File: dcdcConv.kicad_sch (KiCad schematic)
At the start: 72 parts, among them J17 PWRSWITCH, J18 Conn_01x02, J19 EN, J20 Conn_01x03, J21 PGOOD, J22 Conn_01x03, U10 TLV62130, U7 TLV62130, U8 TLV62130, U9 MAX42402AFLB+

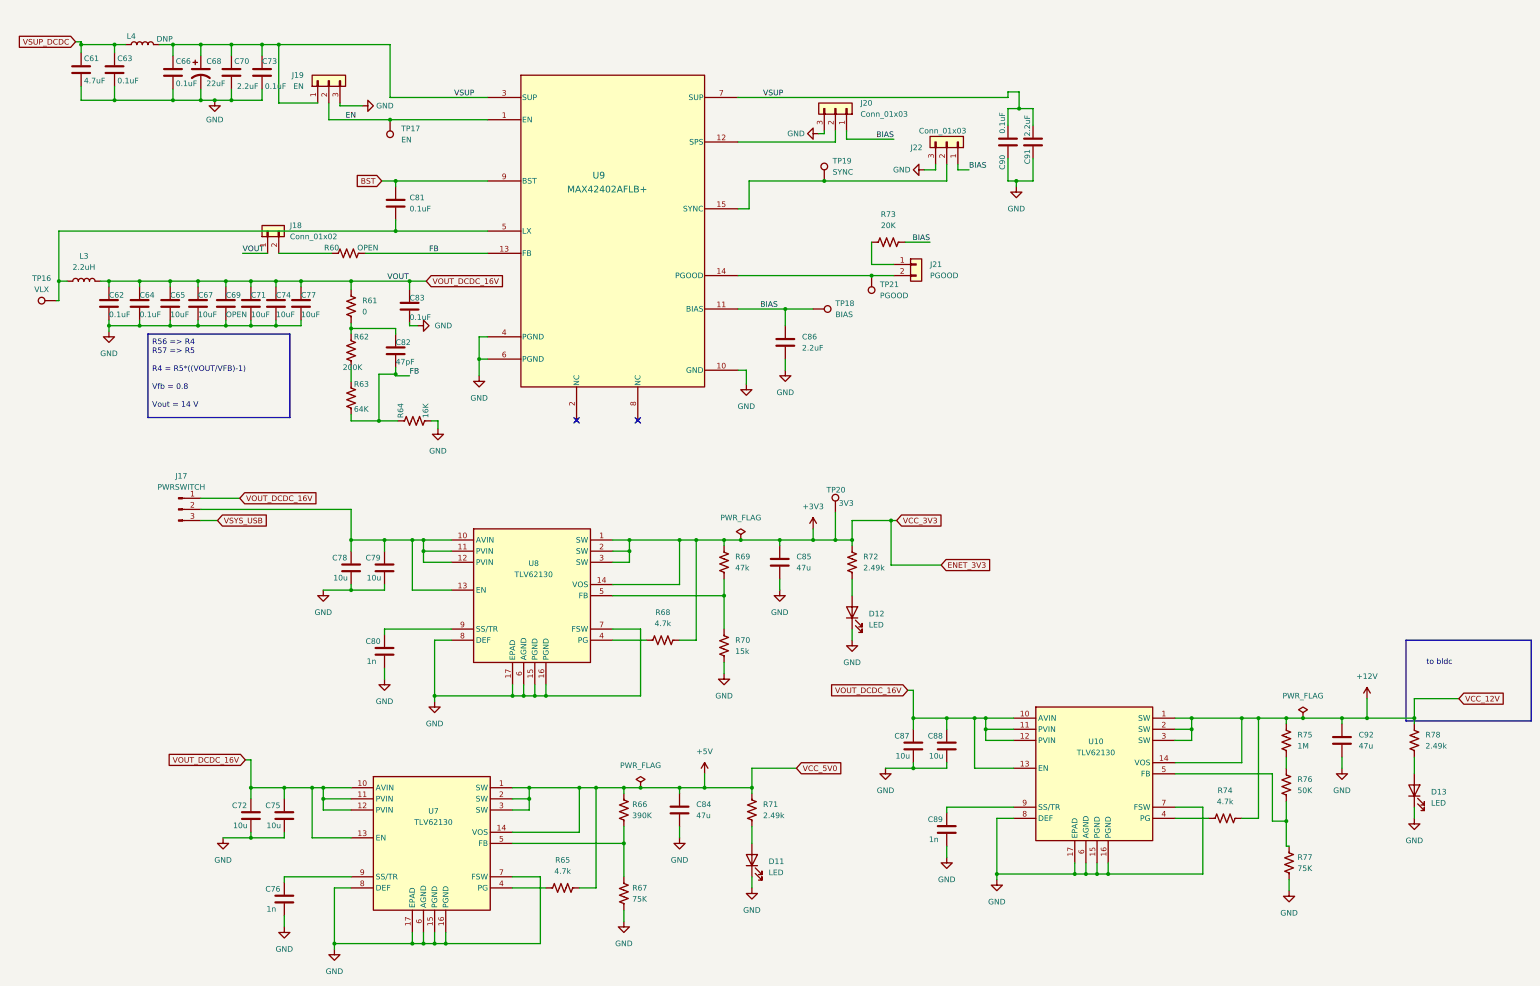
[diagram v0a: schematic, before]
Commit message: dad
da
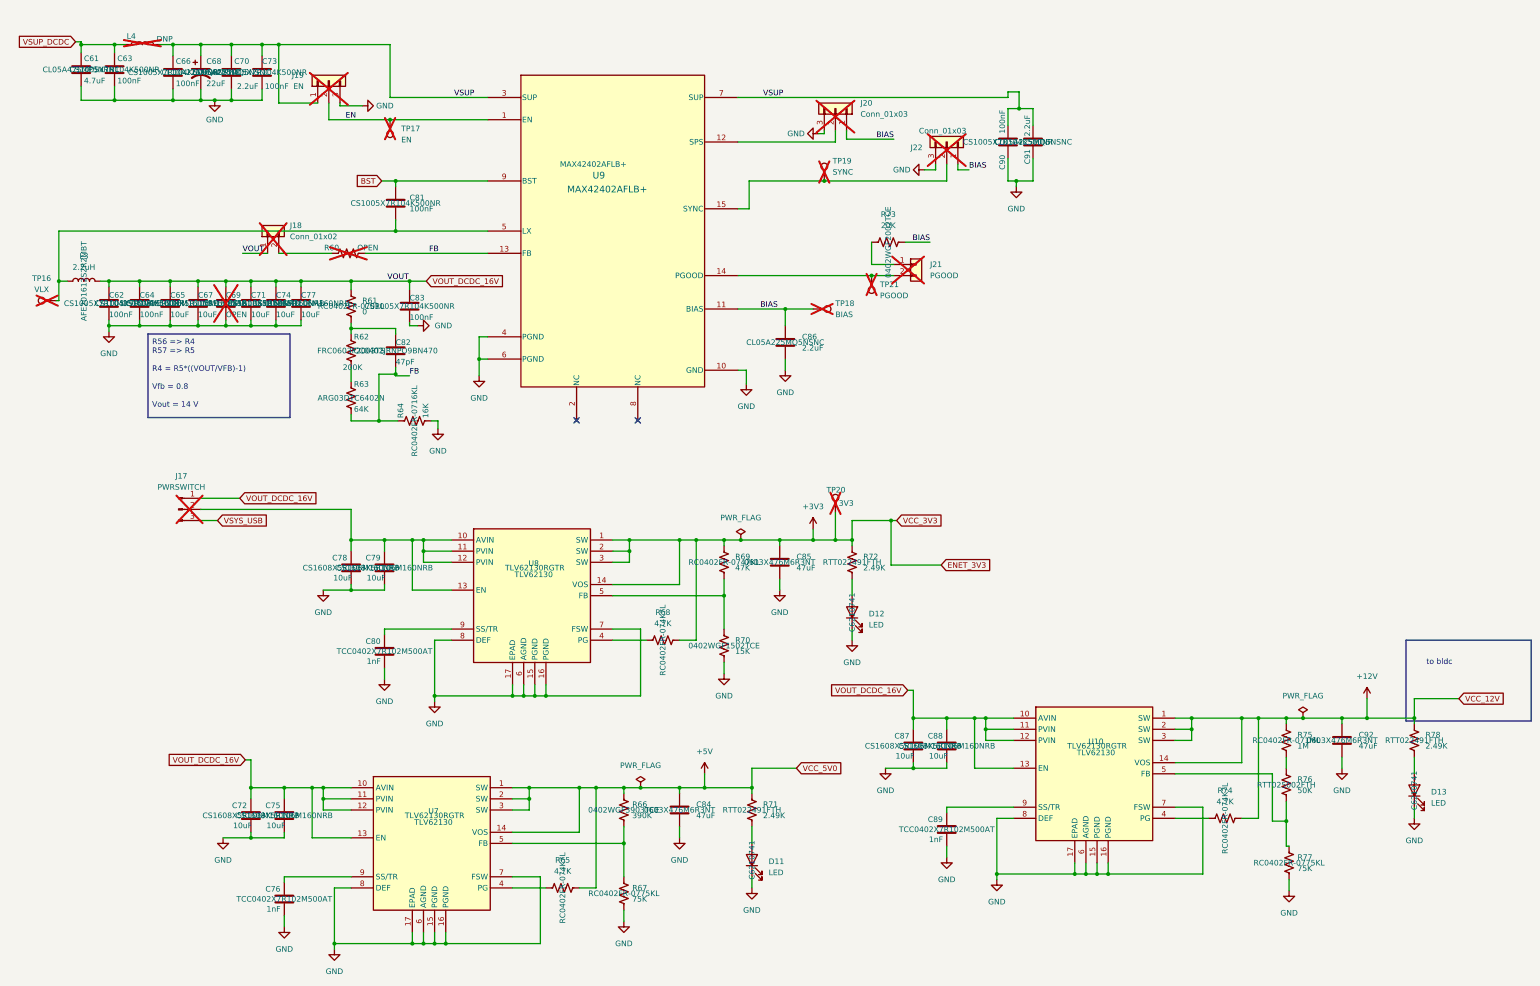
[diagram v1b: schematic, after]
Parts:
- C61: Manufacturer_Part_Number (none) -> CL05A475MP5NRNC
- C62, C63, C64, C66, C73, C81, C83, C90: value 0.1uF -> 100nF; Manufacturer_Part_Number (none) -> CS1005X7R104K500NR
- C65, C67, C71, C74, C77: Manufacturer_Part_Number (none) -> CS1608X5R106M160NRB
- C68: Manufacturer_Part_Number (none) -> CL10A226MQ8NRNC
- C69, J17, J18, J19, J20, J21, J22, L4, R60, TP16, TP17, TP18, TP19, TP20, TP21: now not fitted
- C70, C86, C91: Manufacturer_Part_Number (none) -> CL05A225MQ5NSNC
- C72, C75, C78, C79, C87, C88: value 10u -> 10uF; Manufacturer_Part_Number (none) -> CS1608X5R106M160NRB
- C76, C80, C89: value 1n -> 1nF; Manufacturer_Part_Number (none) -> TCC0402X7R102M500AT
- C82: Manufacturer_Part_Number (none) -> CC0402JRNPO9BN470
- C84, C85, C92: value 47u -> 47uF; Manufacturer_Part_Number (none) -> 0603X476M6R3NT
- D11, D12, D13: Manufacturer_Part_Number (none) -> C6210741
- L3: Manufacturer_Part_Number (none) -> AFE201612S2R2MBT
- R61: Manufacturer_Part_Number (none) -> RC0402FR-070RL
- R62: Manufacturer_Part_Number (none) -> FRC0603F2003TS
- R63: Manufacturer_Part_Number (none) -> ARG03DTC6402N
- R64: Manufacturer_Part_Number (none) -> RC0402FR-0716KL
- R65, R68, R74: value 4.7k -> 4.7K; Manufacturer_Part_Number (none) -> RC0402FR-074K7L
- R66: Manufacturer_Part_Number (none) -> 0402WGF3903TCE
- R67, R77: Manufacturer_Part_Number (none) -> RC0402FR-0775KL
- R69: value 47k -> 47K; Manufacturer_Part_Number (none) -> RC0402FR-0747KL
- R70: value 15k -> 15K; Manufacturer_Part_Number (none) -> 0402WGF1502TCE
- R71, R72, R78: value 2.49k -> 2.49K; Manufacturer_Part_Number (none) -> RTT022491FTH
- R73: Manufacturer_Part_Number (none) -> 0402WGF2002TCE
- R75: Manufacturer_Part_Number (none) -> RC0402FR-071ML
- R76: Manufacturer_Part_Number (none) -> RTT025002FTH
- U10, U7, U8: Manufacturer_Part_Number (none) -> TLV62130RGTR
- U9: Manufacturer_Part_Number (none) -> MAX42402AFLB+

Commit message: gema
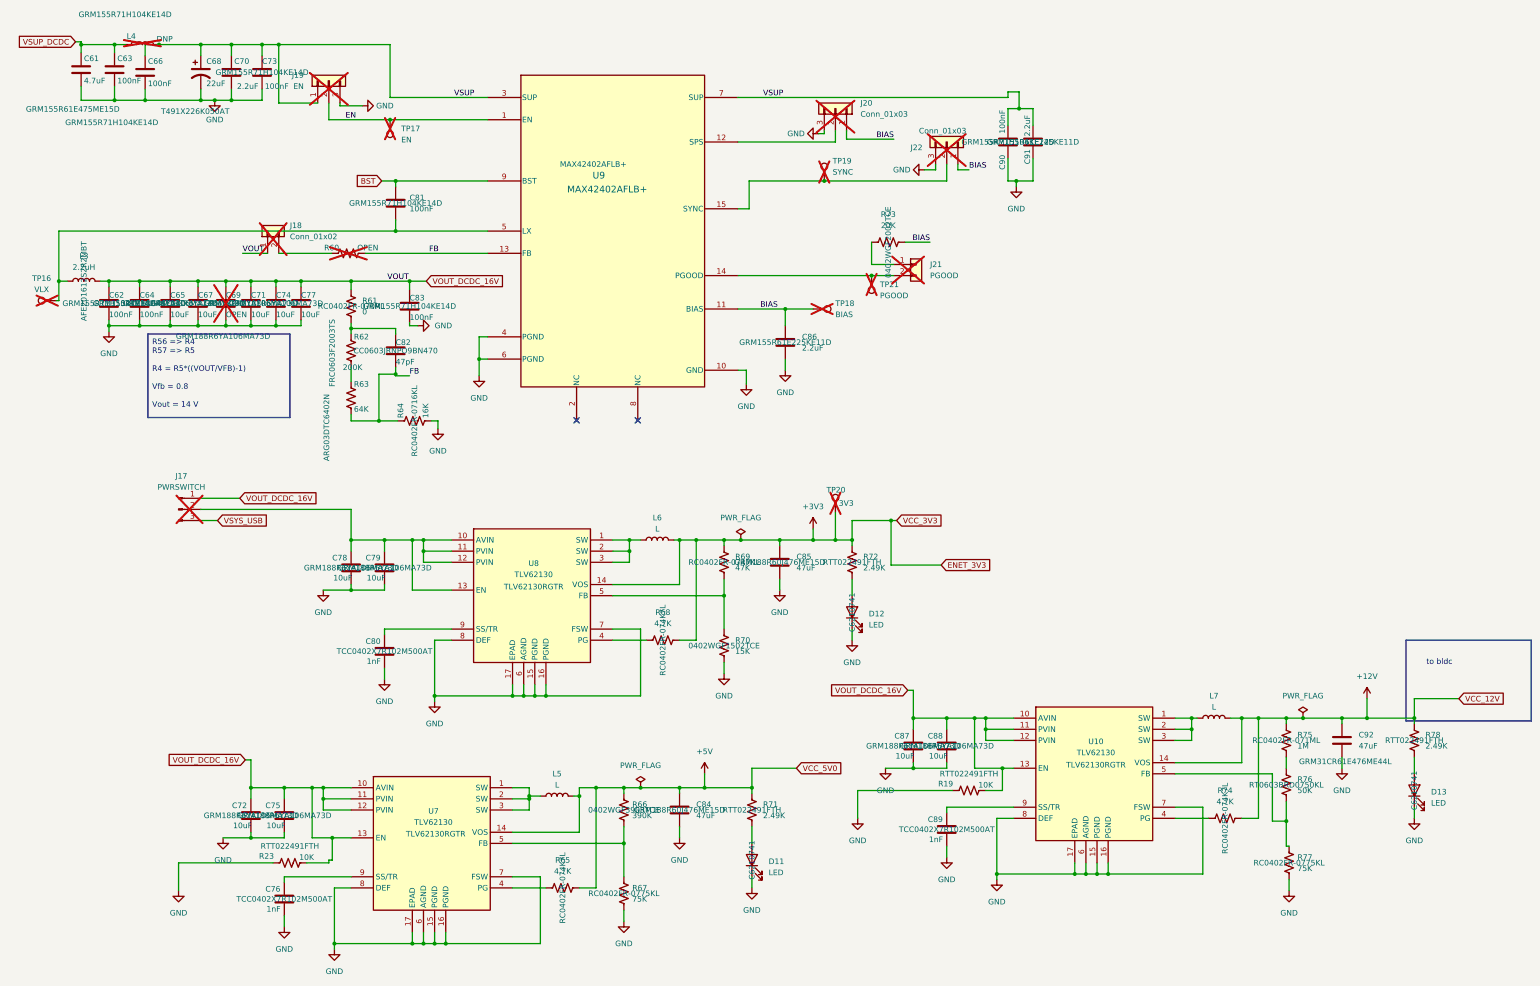
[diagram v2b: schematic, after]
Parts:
- added L5, L6, L7: L, symbol Device:L
- added R19, R23: 10K, Resistor_SMD:R_0402_1005Metric, symbol Device:R_US
- C61:  LCSC Part # (none) -> C2858031; Manufacturer_Part_Number CL05A475MP5NRNC -> GRM155R61E475ME15D
- C62, C63, C64, C66, C73, C81, C83, C90:  LCSC Part # (none) -> C77020; Manufacturer_Part_Number CS1005X7R104K500NR -> GRM155R71H104KE14D
- C65, C67, C71, C72, C74, C75, C77, C78, C79, C87, C88:  LCSC Part # (none) -> C194427; Manufacturer_Part_Number CS1608X5R106M160NRB -> GRM188R6YA106MA73D
- C68: footprint Capacitor_SMD:C_0603_1608Metric -> footprints:CAP-SMD_L7.3-W4.3-R-RD;  LCSC Part # (none) -> C696800; Manufacturer_Part_Number CL10A226MQ8NRNC -> T491X226K050AT
- C70, C86, C91:  LCSC Part # (none) -> C385032; Manufacturer_Part_Number CL05A225MQ5NSNC -> GRM155R61E225KE11D
- C76, C80, C89:  LCSC Part # (none) -> C696907
- C82:  LCSC Part # (none) -> C105622; Manufacturer_Part_Number CC0402JRNPO9BN470 -> CC0603JRNPO9BN470
- C84, C85:  LCSC Part # (none) -> C140782; Manufacturer_Part_Number 0603X476M6R3NT -> GRM188R60J476ME15D
- C92: footprint Capacitor_SMD:C_0603_1608Metric -> Capacitor_SMD:C_1206_3216Metric;  LCSC Part # (none) -> C403725; Manufacturer_Part_Number 0603X476M6R3NT -> GRM31CR61E476ME44L
- D11, D12, D13:  LCSC Part # (none) -> C6210741
- L3:  LCSC Part # (none) -> C41347750
- R61:  LCSC Part # (none) -> C106231
- R62:  LCSC Part # (none) -> C2907009
- R63:  LCSC Part # (none) -> C2902643
- R64:  LCSC Part # (none) -> C163487
- R65, R68, R74:  LCSC Part # (none) -> C105871
- R66:  LCSC Part # (none) -> C25782
- R67, R77:  LCSC Part # (none) -> C137935
- R69:  LCSC Part # (none) -> C93943
- R70:  LCSC Part # (none) -> C25756
- R71, R72, R78:  LCSC Part # (none) -> C102924
- R73:  LCSC Part # (none) -> C25765
- R75:  LCSC Part # (none) -> C138033
- R76: footprint Resistor_SMD:R_0402_1005Metric -> Resistor_SMD:R_0603_1608Metric;  LCSC Part # (none) -> C861451; Manufacturer_Part_Number RTT025002FTH -> RT0603BRD0750KL
- U10, U7, U8:  LCSC Part # (none) -> C122479
- U9:  LCSC Part # (none) -> C22392296
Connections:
- net +12V: now also L7.2; no longer U10.1 (SW), U10.2 (SW), U10.3 (SW)
- net +3V3: now also L6.2; no longer U8.1 (SW), U8.2 (SW), U8.3 (SW)
- net +5V: now also L5.2; no longer U7.1 (SW), U7.2 (SW), U7.3 (SW)
- net GND: now also R19.2, R23.2
- net VOUT_DCDC_16V: now also R19.1, R23.1
- new net: L7.1, U10.1 (SW), U10.2 (SW), U10.3 (SW)
- new net: L5.1, U7.1 (SW), U7.2 (SW), U7.3 (SW)
- new net: L6.1, U8.1 (SW), U8.2 (SW), U8.3 (SW)
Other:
- moved on the sheet: C66
